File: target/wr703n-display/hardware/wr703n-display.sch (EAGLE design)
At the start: 24 parts, among them IC1 MEGA48-AI, J2 22-05-7048-04, J3 22-05-7028-02

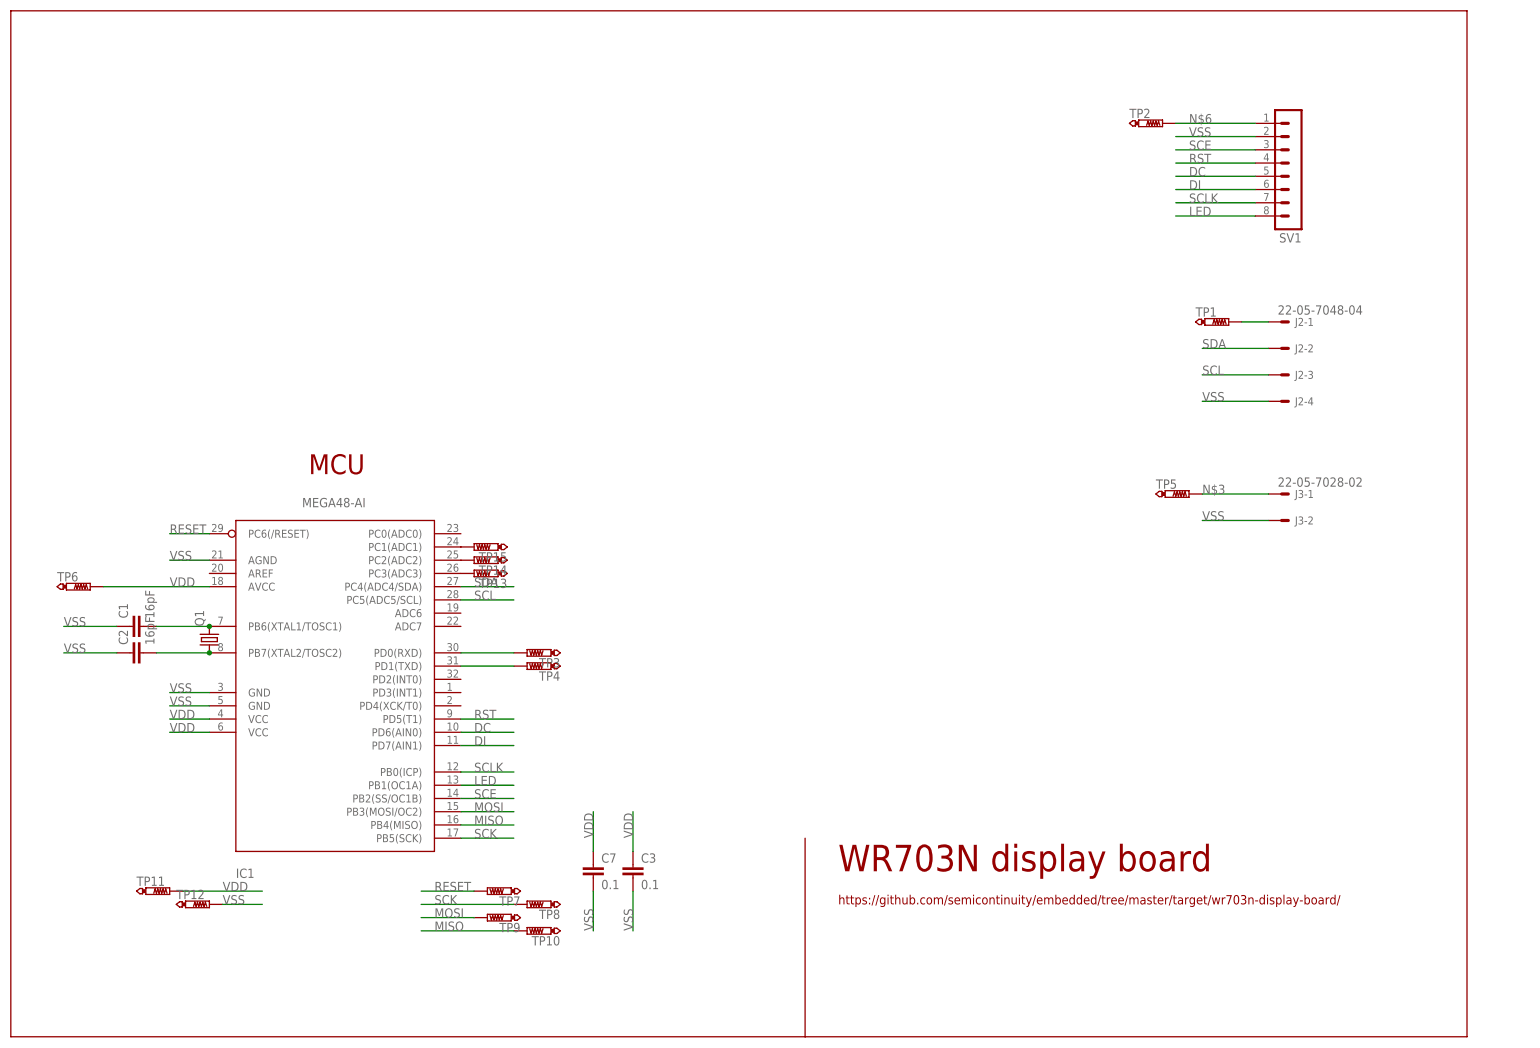
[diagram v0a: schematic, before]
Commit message: wr703n-display
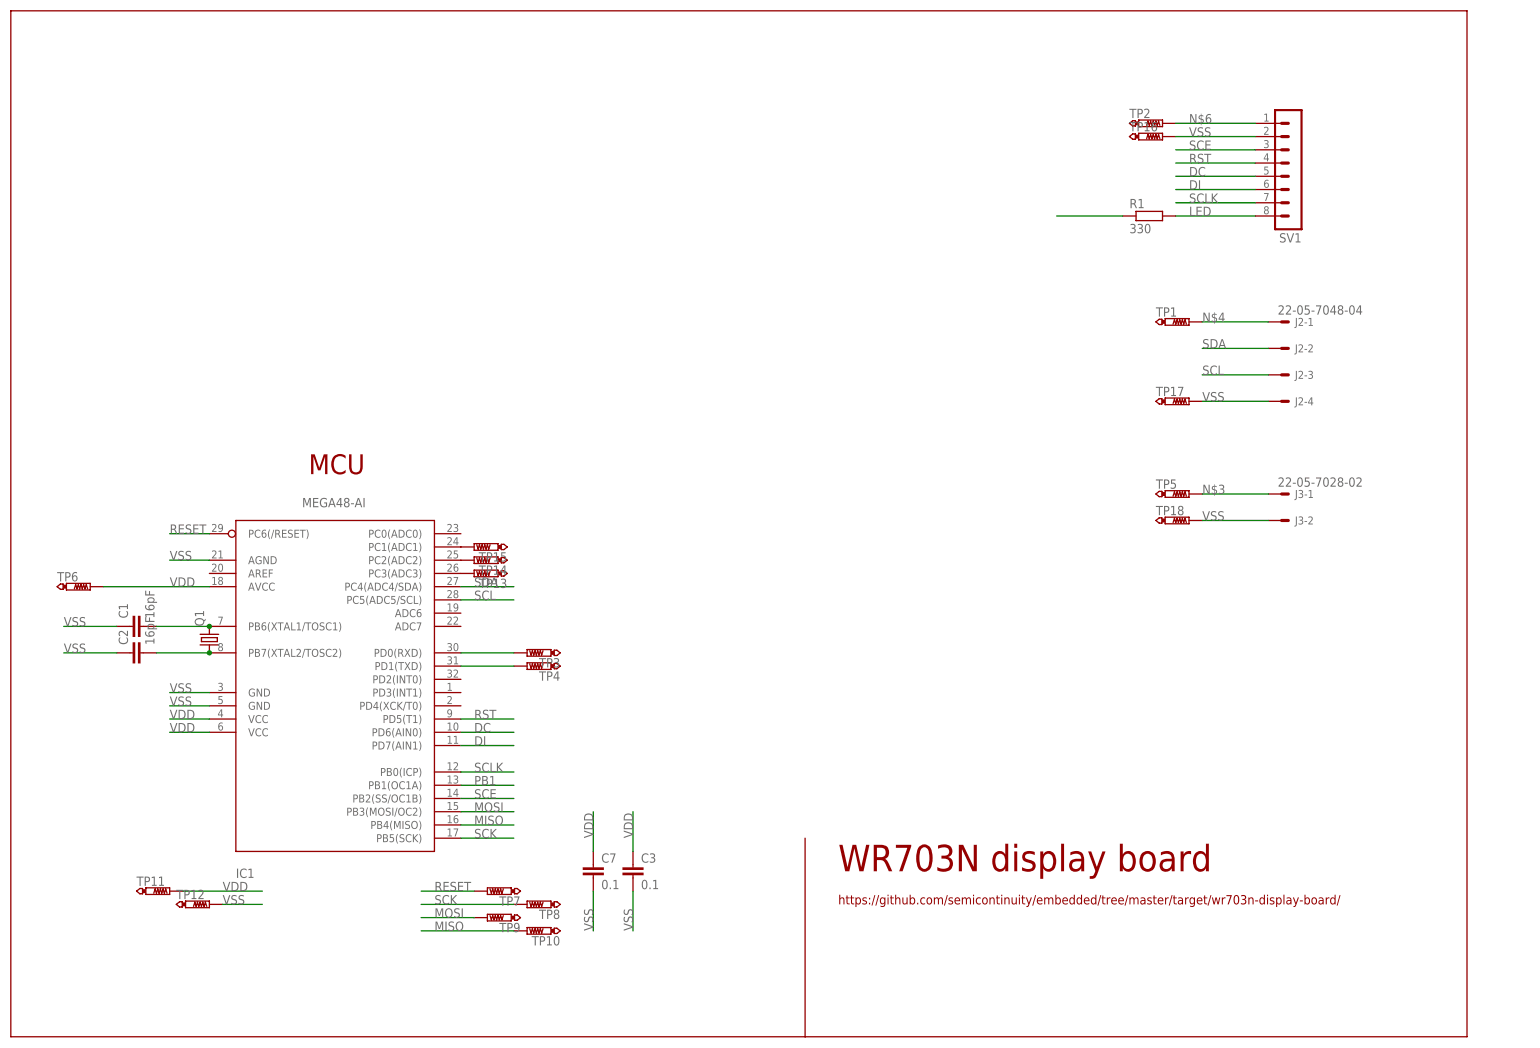
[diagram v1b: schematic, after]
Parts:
- added R1: 330, rcl:R-EU_R0805
- added TP16, TP17, TP18: PTR1B2,54, testpad:PTR1B2,54
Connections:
- new net PB1: IC1.PB1(OC1A), R1.1
- net LED: now also R1.2; no longer IC1.PB1(OC1A)
- net VSS: now also TP16.TP, TP17.TP, TP18.TP
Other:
- moved on the sheet: TP1
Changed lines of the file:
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@@
 <part name="TP15" library="testpad" deviceset="PTR1" device="TP17R"/>
 <part name="C3" library="rcl" deviceset="C-EU" device="C0805" value="0.1"/>
+<part name="TP16" library="testpad" deviceset="PTR1" device="B2,54"/>
+<part name="TP17" library="testpad" deviceset="PTR1" device="B2,54"/>
+<part name="TP18" library="testpad" deviceset="PTR1" device="B2,54"/>
+<part name="R1" library="rcl" deviceset="R-EU_" device="R0805" value="330"/>
 </parts>
 <sheets>
@@
 <instance part="C1" gate="G$1" x="22.86" y="78.74" rot="R90"/>
 <instance part="C2" gate="G$1" x="22.86" y="73.66" rot="R90"/>
-<instance part="TP1" gate="G$1" x="233.68" y="137.16" rot="R270"/>
+<instance part="TP1" gate="G$1" x="226.06" y="137.16" rot="R270"/>
 <instance part="TP3" gate="G$1" x="99.06" y="73.66" rot="R90"/>
 <instance part="TP4" gate="G$1" x="99.06" y="71.12" rot="R90"/>
@@
 <instance part="TP15" gate="G$1" x="88.9" y="93.98" rot="R90"/>
 <instance part="C3" gate="G$1" x="119.38" y="33.02"/>
+<instance part="TP16" gate="G$1" x="220.98" y="172.72" rot="R270"/>
+<instance part="TP17" gate="G$1" x="226.06" y="121.92" rot="R270"/>
+<instance part="TP18" gate="G$1" x="226.06" y="99.06" rot="R270"/>
+<instance part="R1" gate="G$1" x="218.44" y="157.48"/>
 </instances>
 <busses>
@@
 <wire x1="238.76" y1="172.72" x2="223.52" y2="172.72" width="0.1524" layer="91"/>
 <label x="226.06" y="172.72" size="1.778" layer="95"/>
+<pinref part="TP16" gate="G$1" pin="TP"/>
 </segment>
 <segment>
@@
 <label x="228.6" y="121.92" size="1.778" layer="95"/>
 <wire x1="241.3" y1="121.92" x2="228.6" y2="121.92" width="0.1524" layer="91"/>
+<pinref part="TP17" gate="G$1" pin="TP"/>
 </segment>
 <segment>
@@
 <wire x1="241.3" y1="99.06" x2="228.6" y2="99.06" width="0.1524" layer="91"/>
 <label x="228.6" y="99.06" size="1.778" layer="95"/>
+<pinref part="TP18" gate="G$1" pin="TP"/>
 </segment>
 <segment>
@@
 <wire x1="238.76" y1="157.48" x2="223.52" y2="157.48" width="0.1524" layer="91"/>
 <label x="226.06" y="157.48" size="1.778" layer="95"/>
-</segment>
-<segment>
-<pinref part="IC1" gate="G$1" pin="PB1(OC1A)"/>
-<wire x1="86.36" y1="48.26" x2="96.52" y2="48.26" width="0.1524" layer="91"/>
-<label x="88.9" y="48.26" size="1.778" layer="95"/>
+<pinref part="R1" gate="G$1" pin="2"/>
 </segment>
 </net>
@@
 <pinref part="J2" gate="-1" pin="S"/>
 <pinref part="TP1" gate="G$1" pin="TP"/>
-<wire x1="236.22" y1="137.16" x2="241.3" y2="137.16" width="0.1524" layer="91"/>
+<wire x1="228.6" y1="137.16" x2="241.3" y2="137.16" width="0.1524" layer="91"/>
+<label x="228.6" y="137.16" size="1.778" layer="95"/>
 </segment>
 </net>
@@
 </segment>
 </net>
+<net name="PB1" class="0">
+<segment>
+<pinref part="IC1" gate="G$1" pin="PB1(OC1A)"/>
+<wire x1="86.36" y1="48.26" x2="96.52" y2="48.26" width="0.1524" layer="91"/>
+<label x="88.9" y="48.26" size="1.778" layer="95"/>
+</segment>
+<segment>
+<pinref part="R1" gate="G$1" pin="1"/>
+<wire x1="213.36" y1="157.48" x2="200.66" y2="157.48" width="0.1524" layer="91"/>
+</segment>
+</net>
